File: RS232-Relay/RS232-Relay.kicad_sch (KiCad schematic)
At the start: 27 parts, among them J1 Conn_01x08, J2 Conn_01x02, J3 Conn_01x08, J4 Conn_01x09, J5 Conn_01x09, J6 Conn_01x08, J7 Conn_01x03, K1 G5V-1, Q1 2N3904, SW1 SW_SPST, U1 TEC2-1210WI, U2 4N25, U3 MAX3232, U4 MAX3232

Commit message: Basic schematic fully complete
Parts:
- removed C3, C4: 10u, Capacitor_SMD:C_0603_1608Metric, symbol Device:C_Small
- removed C5: 1u, Capacitor_SMD:C_0402_1005Metric, symbol Device:C_Small
- removed SW1: SW_SPST, Switch:PTS841, symbol Switch:SW_SPST
- removed U3: MAX3232, symbol Interface_UART:MAX3232
- added C10, C11, C13, C6, C8, C9: 0.1uF, Capacitor_SMD:C_0402_1005Metric, symbol Device:C_Small
- added C12, C14, C15, C7: 1uF, Capacitor_SMD:C_0402_1005Metric, symbol Device:C_Small
- added D3, D4: WS2812B, LED_SMD:LED_WS2812B_PLCC4_5.0x5.0mm_P3.2mm, symbol LED:WS2812B
- added D5, D6, D7: Green, LED_SMD:LED_0805_2012Metric, symbol Device:LED
- added J8: RS232_2, Connector_Phoenix_MSTB:PhoenixContact_MSTBA_2,5_3-G-5,08_1x03_P5.08mm_Horizontal, symbol Connector_Generic:Conn_01x03
- added R10: 50R, Resistor_SMD:R_0603_1608Metric, symbol Device:R_US
- added R6, R7: 10K, Resistor_SMD:R_0402_1005Metric, symbol Device:R_US
- added R8: 4K7, Resistor_SMD:R_0603_1608Metric, symbol Device:R_US
- added R9: 220R, Resistor_SMD:R_0603_1608Metric, symbol Device:R_US
- added SW2, SW3: SW_SPST, Switch:PTS841, symbol Switch:SW_SPST
- added TP1: 3V3, TestPoint:TestPoint_Pad_D1.0mm, symbol Connector:TestPoint
- added TP10: I2C_SCL, TestPoint:TestPoint_Pad_D1.0mm, symbol Connector:TestPoint
- added TP11: I2C_INT, TestPoint:TestPoint_Pad_D1.0mm, symbol Connector:TestPoint
- added TP12: BTN_01, TestPoint:TestPoint_Pad_D1.0mm, symbol Connector:TestPoint
- added TP13: BTN_02, TestPoint:TestPoint_Pad_D1.0mm, symbol Connector:TestPoint
- added TP2: Signal In, TestPoint:TestPoint_Pad_D1.0mm, symbol Connector:TestPoint
- added TP3: Signal Out, TestPoint:TestPoint_Pad_D1.0mm, symbol Connector:TestPoint
- added TP4: GND_ISO, TestPoint:TestPoint_Pad_D1.0mm, symbol Connector:TestPoint
- added TP5: UART_1_TX, TestPoint:TestPoint_Pad_D1.0mm, symbol Connector:TestPoint
- added TP6: UART_1_RX, TestPoint:TestPoint_Pad_D1.0mm, symbol Connector:TestPoint
- added TP7: UART_2_TX, TestPoint:TestPoint_Pad_D1.0mm, symbol Connector:TestPoint
- added TP8: UART_2_RX, TestPoint:TestPoint_Pad_D1.0mm, symbol Connector:TestPoint
- added TP9: I2C_SDA, TestPoint:TestPoint_Pad_D1.0mm, symbol Connector:TestPoint
- added U3: PCF8575DBR, Package_SO:SSOP-24_5.3x8.2mm_P0.65mm, symbol Interface_Expansion:PCF8575DBR
- added U5: LTV-847S, Package_DIP:SMDIP-16_W9.53mm, symbol Isolator:LTV-847S
- C1, C2: value 47u -> 10u; footprint Capacitor_SMD:C_1206_3216Metric -> Capacitor_SMD:C_0603_1608Metric; LCSC C96123 -> C19702
- D1: value D -> 1N4148W
- D2: value LED -> RED
- F1: now not fitted; now left out of the parts list
- J1: value Conn_01x08 -> Relay 1-4
- J3: value Conn_01x08 -> Relay 5-8
- J6: value Conn_01x08 -> Relay 9-12
- J7: value Conn_01x03 -> RS232_1; footprint (none) -> Connector_Phoenix_MSTB:PhoenixContact_MSTBA_2,5_3-G-5,08_1x03_P5.08mm_Horizontal
- R1: value 470R -> 1000R; LCSC C23179 -> C21190
- R2: value 330R -> 1000R; LCSC C23138 -> C21190
- R4: value 10K -> 4K7; footprint Resistor_SMD:R_0402_1005Metric -> Resistor_SMD:R_0603_1608Metric; LCSC C25744 -> C23162
- U4: footprint (none) -> Package_SO:TSSOP-16_4.4x5mm_P0.65mm
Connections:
- net ESP_BTN_01 is gone; now on net +3V3: R4.2
- net IN_01 is gone; now on net +12V: R1.1
- net +12V: now also C2.1, J2.1 (Pin_1); no longer F1.2
- net +3V3: now also U4.16 (VCC), C12.2, C13.2, C7.2, C9.2, R10.2, R6.1, R7.1, R8.1, TP1.1, U3.24 (VCC); no longer C2.1, R4.1
- net +5V: now also D3.1 (VDD), D4.1 (VDD), R9.2
- net ESP32_GPIO_01: now also D3.4 (DIN)
- net ESP32_GPIO_03: now also R8.2, TP9.1, U3.23 (SDA)
- net ESP32_GPIO_04: now also R4.1, TP10.1, U3.22 (SCL)
- net ESP32_GPIO_05: now also TP11.1, U3.1 (~{INT})
- net ESP32_GPIO_14: now also U4.10 (T2IN), TP7.1
- net ESP32_GPIO_15: now also U4.9 (R2OUT), TP8.1
- net ESP32_UART0_RX: now also U4.12 (R1OUT), TP6.1
- net ESP32_UART0_TX: now also U4.11 (T1IN), TP5.1
- net GND: now also C2.2, D5.1 (K)
- net GNDREF: now also J7.3 (Pin_3), U4.15 (GND), C10.1, C11.1, C12.1, C13.1, C14.1, C15.1, C7.1, C9.1, D3.3 (VSS), D4.3 (VSS), D6.1 (K), D7.1 (K), J8.3 (Pin_3), SW2.2 (B), SW3.2 (B), TP4.1, U3.12 (GND), U3.2 (A1), U3.21 (A0), U3.3 (A2); no longer C2.2
- net RELAY_01: now also TP3.1
- net at R1.2: now also D5.2 (A); no longer U2.1
- net RS232_1_TX: now reaches J7.1 (Pin_1)
- net RS232_1_TX: now also U4.14 (T1OUT)
- net RS232_1_RX: now reaches J7.2 (Pin_2)
- net RS232_1_RX: now also U4.13 (R1IN)
- net at R5.1: now also U2.1
- net RELAY_IN_01: now reaches R5.2
- net RELAY_IN_01: now also TP2.1, U3.4 (P0)
- net at F1.1: no longer J2.1 (Pin_1)
- net at U4.1 (C1+): now also C6.1
- net at U4.2 (VS+): now also C11.2
- net at U4.3 (C1-): now also C6.2
- net at U4.4 (C2+): now also C8.2
- net at U4.5 (C2-): now also C8.1
- net at U4.6 (VS-): now also C10.2
- net RS232_2_TX: now reaches U4.7 (T2OUT)
- net RS232_2_TX: now also J8.1 (Pin_1)
- net RS232_2_RX: now reaches U4.8 (R2IN)
- net RS232_2_RX: now also J8.2 (Pin_2)
- net ESP32_GPIO_21 renamed BTN_01
- net BTN_01: now also C14.2, R6.2, SW2.1 (A), TP12.1
- net ESP32_GPIO_22 renamed BTN_02
- net BTN_02: now also C15.2, R7.2, SW3.1 (A), TP13.1
- new net: D3.2 (DOUT), D4.4 (DIN)
- new net: D6.2 (A), R10.1
- new net: D7.2 (A), R9.1
- new net RELAY_IN_02: U3.5 (P1)
- new net RELAY_IN_03: U3.6 (P2)
- new net RELAY_IN_04: U3.7 (P3)
- new net RELAY_IN_05: U3.8 (P4)
- new net RELAY_IN_06: U3.9 (P5)
- new net RELAY_IN_07: U3.10 (P6)
- new net RELAY_IN_08: U3.11 (P7)
- new net RELAY_IN_09: U3.13 (P10)
- new net RELAY_IN_10: U3.14 (P11)
- new net RELAY_IN_11: U3.15 (P12)
- new net RELAY_IN_12: U3.16 (P13)
- no-connect marks 1 -> 7
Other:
- note added: "10mA"
- note added: "12-3V DC-DC Regulator"
- note added: "12V power input"
- note added: "3.3v isolated from 12v using TEC2-1210WI"
- note added: "3v3 input from IO Expander (PCF8575DBR)"
- note added: "Buttons"
- note added: "How to calculate this value?"
- note added: "I2C Pullup"
- note added: "IO Expansion"
- note added: "If = 25mA (max) If = 10mA (target) Vf = 2V"
- note added: "If = 50mA (max) If = 10mA (target) Vf = 1.3V"
- note added: "Indicator LEDs"
- note added: "MIGRATE TO 5V regulator and use ESP32 onboard"
- note added: "RS232 Isolated Input Driver"
- note added: "Relay Outputs"
- note added: "Relay flips between 0 and 12V for output"
- note added: "Test Points"
- note removed: "3v3 input from ESP32"
- note removed: "Calc this value"
- note removed: "Connect this to ESP32"
- note removed: "Consider if capacitors are needed or left blank"
- note removed: "Test points"
- moved on the sheet: D1, D2, J1, J2, J3, J6, J7, K1, Q1, R3, U1, U2

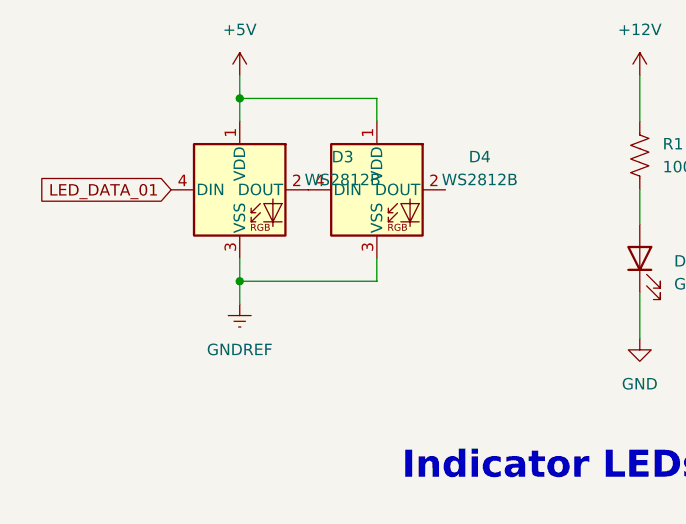
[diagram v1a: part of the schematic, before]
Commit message: Fixing pin headers
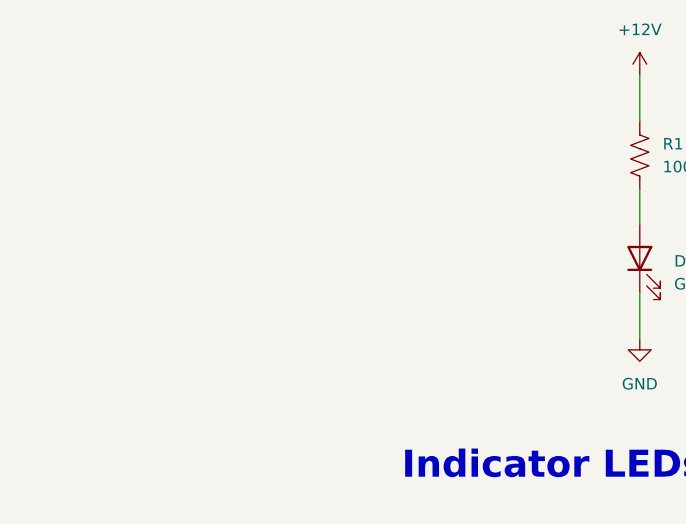
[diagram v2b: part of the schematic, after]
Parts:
- removed D3, D4: WS2812B, LED_SMD:LED_WS2812B_PLCC4_5.0x5.0mm_P3.2mm, symbol LED:WS2812B
- J4, J5: footprint Connector_PinHeader_2.54mm:PinHeader_1x09_P2.54mm_Vertical -> Connector_PinSocket_2.54mm:PinSocket_1x09_P2.54mm_Vertical
